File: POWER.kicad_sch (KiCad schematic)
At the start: 23 parts, among them U1 OPA1644AxD, U2 OPA1612AxD, U3 LT3032-12

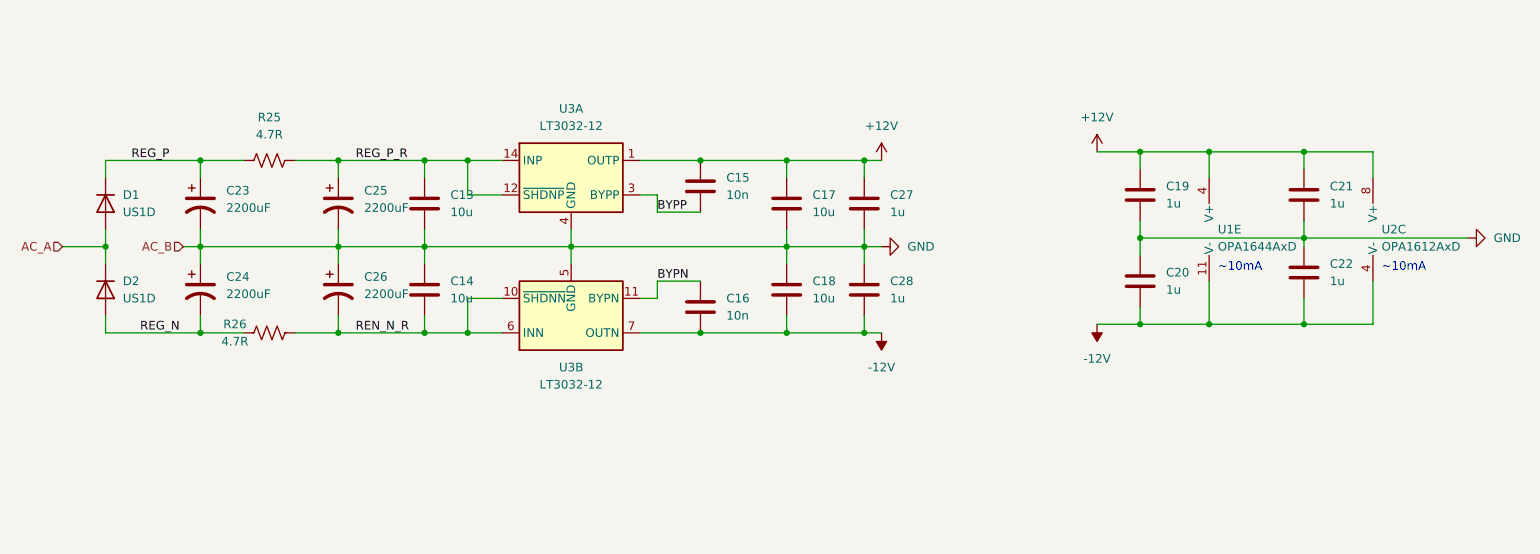
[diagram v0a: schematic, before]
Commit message: CHANGE POWER SUPPLY
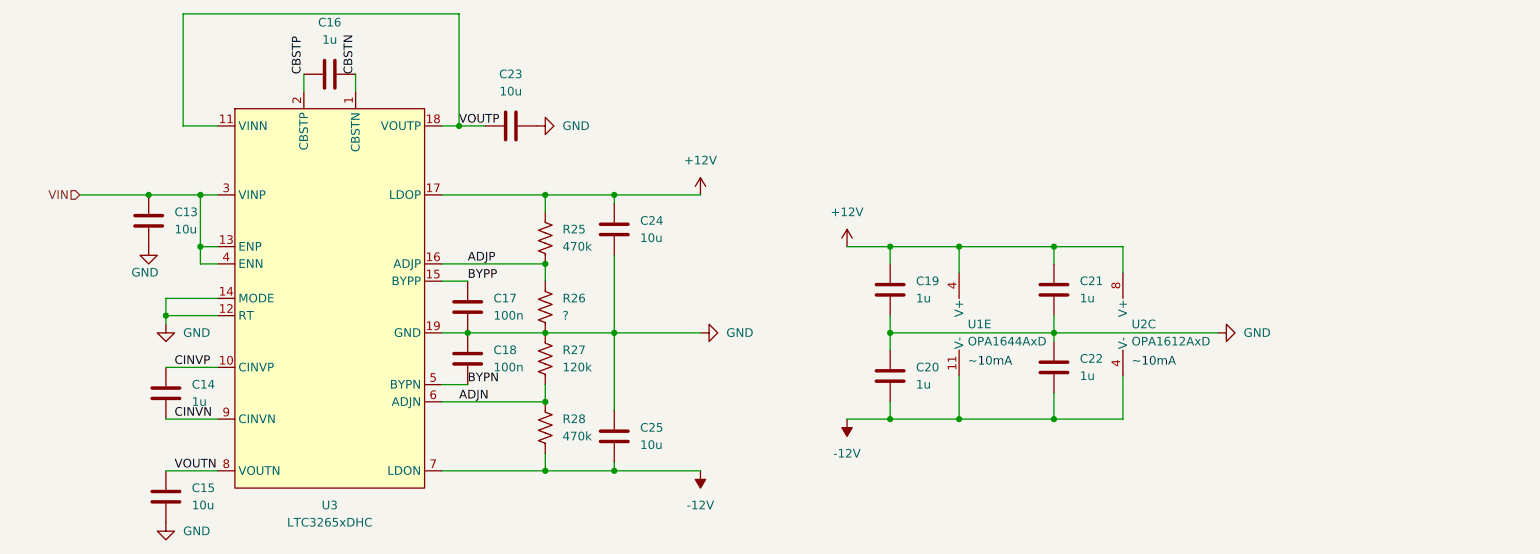
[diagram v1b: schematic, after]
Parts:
- removed C23, C24, C25, C26: 2200uF, Capacitor_SMD:CP_Elec_18x17.5, symbol Device:C_Polarized_US
- removed C27, C28: 1u, Capacitor_SMD:C_0402_1005Metric, symbol Device:C
- removed D1, D2: US1D, Diode_SMD:D_SMA, symbol Diode:US1D
- removed U3: LT3032-12, Package_DFN_QFN:Linear_DE14MA, symbol Regulator_Linear:LT3032-12
- added C23, C24, C25: 10u, Capacitor_SMD:C_0805_2012Metric, symbol Device:C
- added R27: 120k, Resistor_SMD:R_0402_1005Metric, symbol Device:R_US
- added R28: 470k, Resistor_SMD:R_0402_1005Metric, symbol Device:R_US
- added U3: LTC3265xDHC, Package_DFN_QFN:DFN-18-1EP_3x5mm_P0.5mm_EP1.66x4.4mm, symbol OPA_PHONO:LTC3265xDHC
- C14: value 10u -> 1u; footprint Capacitor_SMD:C_0805_2012Metric -> Capacitor_SMD:C_0402_1005Metric
- C15: value 10n -> 10u; footprint Capacitor_SMD:C_0402_1005Metric -> Capacitor_SMD:C_0805_2012Metric
- C16: value 10n -> 1u
- C17, C18: value 10u -> 100n; footprint Capacitor_SMD:C_0805_2012Metric -> Capacitor_SMD:C_0402_1005Metric
- R25: value 4.7R -> 470k; footprint Resistor_SMD:R_2512_6332Metric -> Resistor_SMD:R_0402_1005Metric
- R26: value 4.7R -> ?; footprint Resistor_SMD:R_2512_6332Metric -> Resistor_SMD:R_0402_1005Metric
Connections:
- net REG_P is gone; now on net +12V: R25.1
- net +12V: now also C24.2, U3.17 (LDOP); no longer C15.2, C17.2
- net -12V: now also C25.1, R28.2, U3.7 (LDON); no longer C16.1, C18.1
- net BYPN: now also C18.1, U3.5 (BYPN); no longer C16.2
- net BYPP: now also C17.2, U3.15 (BYPP); no longer C15.1
- net GND: now also C15.1, R26.2, C23.1, C24.1, C25.2, R27.1, U3.12 (RT), U3.14 (MODE), U3.19 (GND); no longer C14.2
- net REG_N renamed ADJP
- net ADJP: now also R25.2, U3.16 (ADJP)
- net REG_P_R renamed VIN
- net VIN: now also U3.13 (ENP), U3.3 (VINP), U3.4 (ENN); no longer R25.2
- net REN_N_R renamed CINVN
- net CINVN: now also U3.9 (CINVN); no longer R26.2
- new net ADJN: R27.2, R28.1, U3.6 (ADJN)
- new net CBSTN: C16.2, U3.1 (CBSTN)
- new net CBSTP: C16.1, U3.2 (CBSTP)
- new net CINVP: C14.2, U3.10 (CINVP)
- new net VOUTN: C15.2, U3.8 (VOUTN)
- new net VOUTP: C23.2, U3.11 (VINN), U3.18 (VOUTP)
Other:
- moved on the sheet: C19, C20, C21, C22, U1E, U2C
